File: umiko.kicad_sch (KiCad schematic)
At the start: 396 parts, among them J1 USB_C_Receptacle_USB2.0, J2 MJ-4PP-9, J3 MJ-4PP-9, J4 USB_C_Receptacle_USB2.0, SW1 SWITCH, SW2 SWITCH, U1 USBLC6-2P6, U10 TLV75533PDQNR, U11 RP2040, U2 TLV75533PDQNR, U3 W25Q128JVPIQ, U5 SN74LVC1T45DRL, U6 W25Q128JVPIQ, U7 RP2040, U8 SN74LVC1T45DRL, U9 USBLC6-2P6, Y1 12MHz, Y2 12MHz

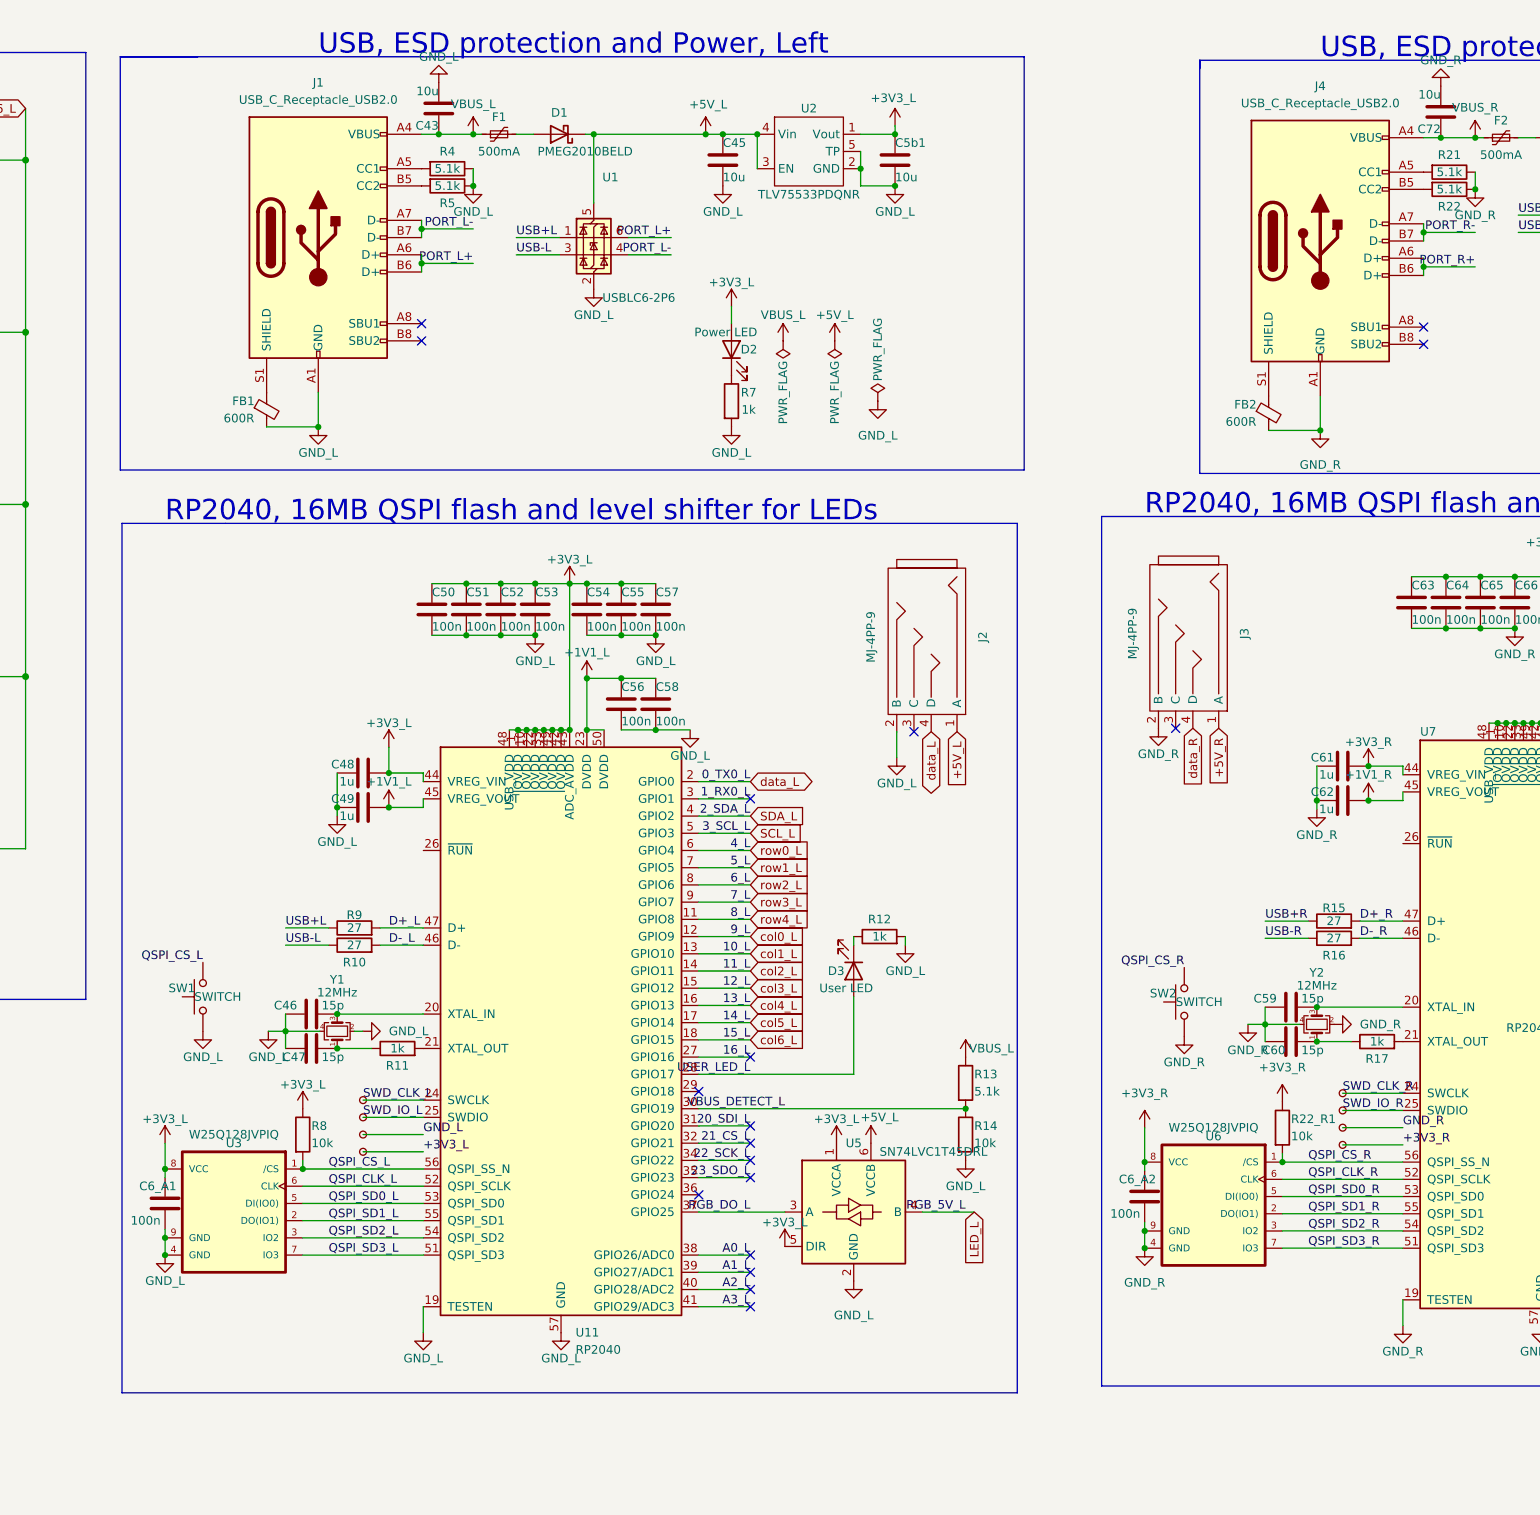
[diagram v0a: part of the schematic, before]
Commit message: Soften corners, clean library refs, drop OLED remnants
- Edge.Cuts corners enlarged to 2mm fillets, then fully unfilleted to
  sharp 90deg in preparation for board squish (both halves still form
  closed loops at 5um tolerance).
- Schematic Footprint property fixed for U2/U3/U6/U10: '0xcb:' prefix
  corrected to 'PCM_0xcb:' so Update PCB from Schematic resolves.
- Removed two orphan Display:ER_OLEDM0.91_1x-I2C footprints (REF**, no
  schematic counterpart) leftover from the dropped OLED design.

Co-Authored-By: Claude Opus 4.7 (1M context) <noreply@anthropic.com>
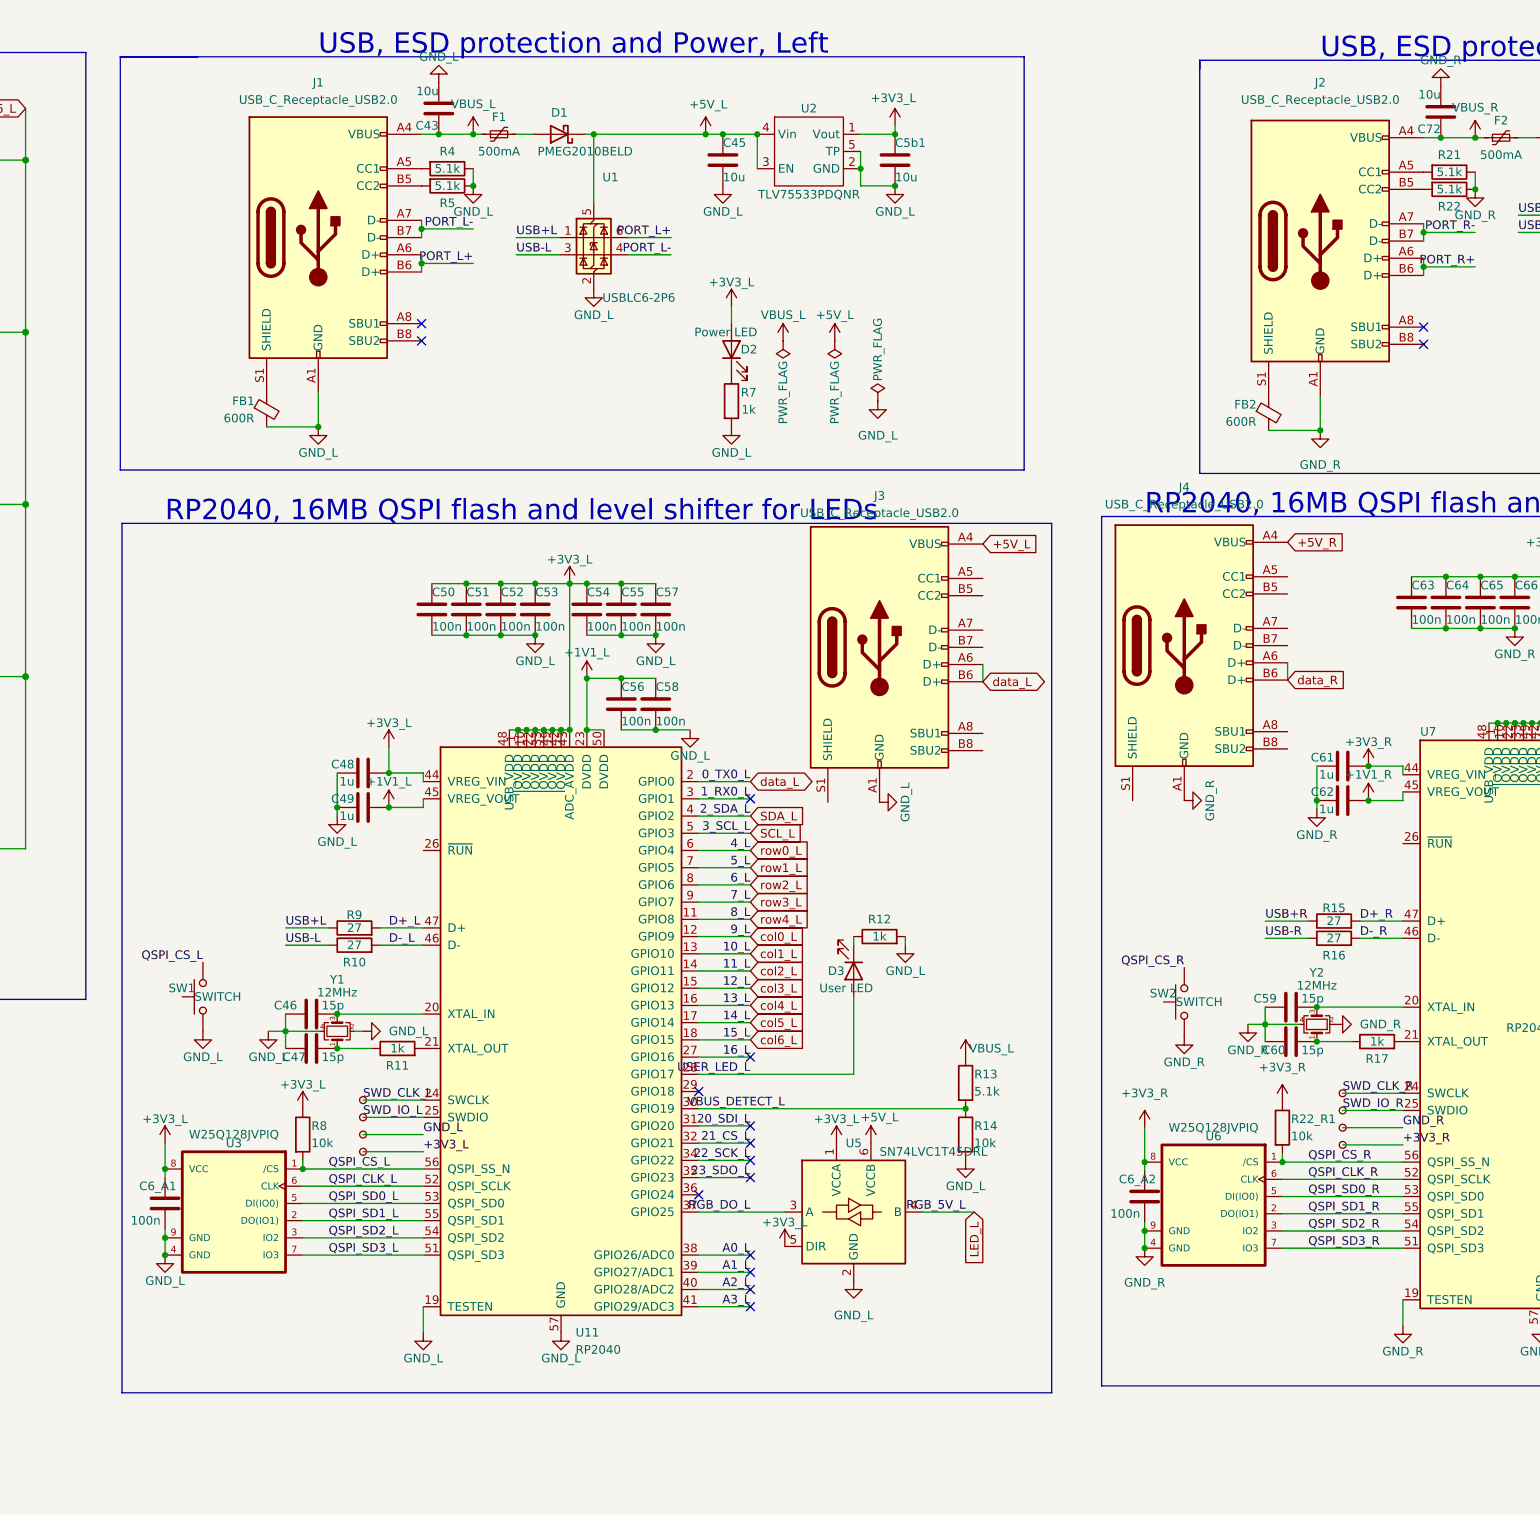
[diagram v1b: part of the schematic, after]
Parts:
- removed J2, J3: MJ-4PP-9, mj-4pp-9:MJ-4PP-9, symbol mj-4pp-9:MJ-4PP-9
- added J3, J4: USB_C_Receptacle_USB2.0, PCM_0xcb:USB_C_Receptacle_HRO_TYPE-C-31-M-12, symbol Connector:USB_C_Receptacle_USB2.0
- U10, U2: footprint 0xcb:X2SON-4 -> PCM_0xcb:X2SON-4
- U3, U6: footprint 0xcb:W25Q128JVPIQ -> PCM_0xcb:W25Q128JVPIQ
- renumbered J4 to J2
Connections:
- net +5V_L: now also J3.A4 (VBUS), J3.A9 (VBUS), J3.B4 (VBUS), J3.B9 (VBUS)
- net +5V_R: now also J4.A4 (VBUS), J4.A9 (VBUS), J4.B4 (VBUS), J4.B9 (VBUS)
- net GND_L: now also J3.A1 (GND), J3.A12 (GND), J3.B1 (GND), J3.B12 (GND)
- net GND_R: now also J4.A1 (GND), J4.A12 (GND), J4.B1 (GND), J4.B12 (GND)
- net data_L: now also J3.A6 (D+), J3.B6 (D+)
- net data_R: now also J4.A6 (D+), J4.B6 (D+)
- no-connect marks 32 -> 30
